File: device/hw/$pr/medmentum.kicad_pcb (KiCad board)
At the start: 2 copper layers, 2 parts, among them U1 BQ27441DRZR-G1B, U2 BQ24074RGTR

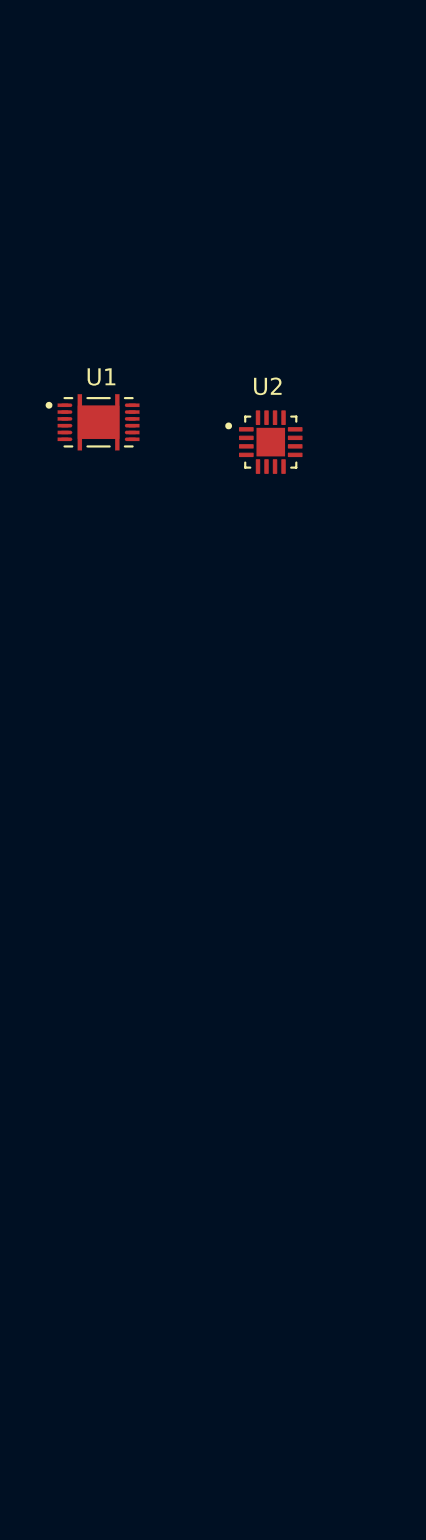
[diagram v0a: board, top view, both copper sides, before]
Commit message: *
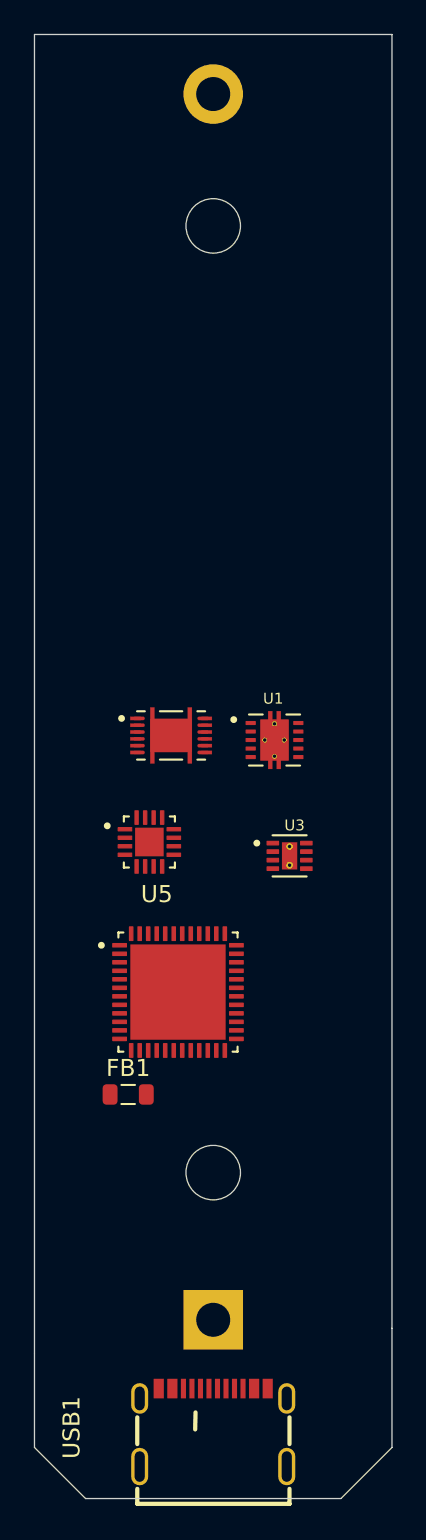
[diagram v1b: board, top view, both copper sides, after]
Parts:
- added BAT1: Battery_Cell, Battery:BatteryHolder_MPD_BH-18650-PC2, B.Cu at (147.0, 133.0)
- added FB1: 100R@100MHz, Inductor_SMD:L_0805_2012Metric, F.Cu at (142.0, 119.8)
- added U3: TPS62082DSGR, fpl:TPS62082DSGR, F.Cu at (151.5, 105.8)
- added U4: BQ27441DRZR-G1B, fpl:BQ27441DRZR-G1B, F.Cu at (144.5, 98.7)
- added U5: STM32F411CEU6, fpl:STM32F411CEU6, F.Cu at (144.9, 113.8)
- added USB1: USB-310F-B-SU, fpl:USB-310F-B-SU, F.Cu at (147.0, 139.3)
- U1: value BQ27441DRZR-G1B -> TPS63002DRCT; footprint fpl:BQ27441DRZR-G1B -> fpl:TPS63002DRCR
- U2: value BQ24074RGTR -> BQ24074RGTR
- moved U2 24.5 mm to (143.2, 104.9)
- moved U1 21.3 mm to (150.6, 98.9)
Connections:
- net /South Bridge/Battery Managment System/VBSIN renamed VBUS
- net Net-(U2-BAT-Pad2) renamed BATSYS
- U1 pad 1: unconnected-(U1-SDA-Pad1) -> BCKOUT5
- U1 pad 10: unconnected-(U1-BIN-Pad10) -> BCKOUT5
- U1 pad 11: (no net) -> GNDD
- U1 pad 12: unconnected-(U1-GPOUT-Pad12) -> (no net)
- U1 pad 13: unconnected-(U1-EXP-Pad13) -> (no net)
- U1 pad 2: unconnected-(U1-SCL-Pad2) -> Net-(U1-L2)
- U1 pad 3: unconnected-(U1-VSS-Pad3) -> GNDD
- U1 pad 4: (no net) -> Net-(U1-L1)
- U1 pad 5: unconnected-(U1-VDD-Pad5) -> BCOUT
- U1 pad 6: unconnected-(U1-BAT-Pad6) -> Net-(U1-EN)
- U1 pad 7: unconnected-(U1-SRN-Pad7) -> Net-(U1-EN)
- U1 pad 8: unconnected-(U1-SRP-Pad8) -> Net-(U1-EN)
- U1 pad 9: (no net) -> GNDD
- U2 pad 1: unconnected-(U2-TS-Pad1) -> /South Bridge/Battery Managment System/TS
- U2 pad 10: /South Bridge/Battery Managment System/BCOUT -> BCOUT
- U2 pad 11: /South Bridge/Battery Managment System/BCOUT -> unconnected-(U2-OUT-Pad11)
- U2 pad 12: unconnected-(U2-ILIM-Pad12) -> /South Bridge/Battery Managment System/ILIM
- U2 pad 14: unconnected-(U2-TMR-Pad14) -> GNDD
- U2 pad 15: unconnected-(U2-ITERM-Pad15) -> /South Bridge/Battery Managment System/ITERM
- U2 pad 16: unconnected-(U2-ISET-Pad16) -> /South Bridge/Battery Managment System/ISET
- U2 pad 4: unconnected-(U2-~{CE}-Pad4) -> /South Bridge/Battery Managment System/CHG_#CE
- U2 pad 5: unconnected-(U2-EN2-Pad5) -> BCOUT
- U2 pad 6: unconnected-(U2-EN1-Pad6) -> GNDD
- U2 pad 7: unconnected-(U2-~{PGOOD}-Pad7) -> /South Bridge/Battery Managment System/CHG_#PGOOD
- U2 pad 9: unconnected-(U2-~{CHG}-Pad9) -> /South Bridge/Battery Managment System/CHG_#CHG
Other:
- board outline added: 21 x 86 mm
